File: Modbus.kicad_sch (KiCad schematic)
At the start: 30 parts, among them J4 Term, J5 RS485, J6 RS422, J7 Term, U5 THVD1452DGSR, U6 THVD1452DGSR

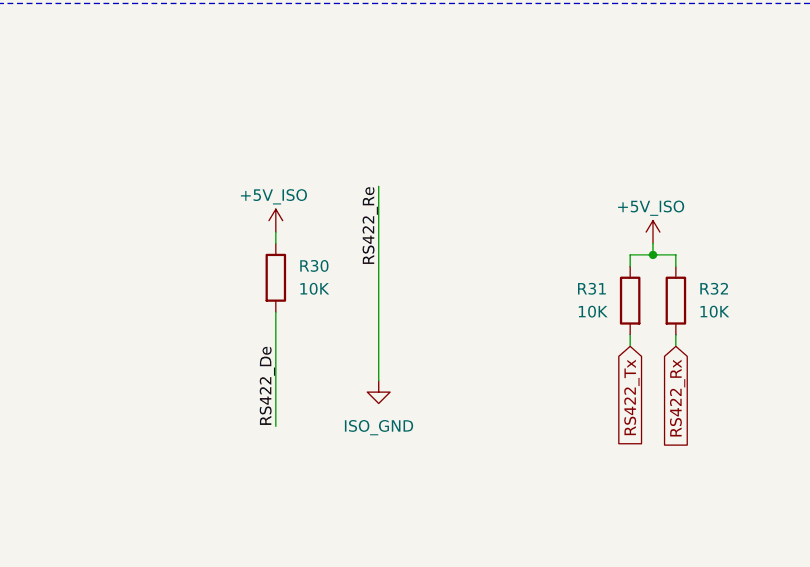
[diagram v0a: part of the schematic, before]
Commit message: reverted back to og files
[local revision r5 4274e03a1d0e]
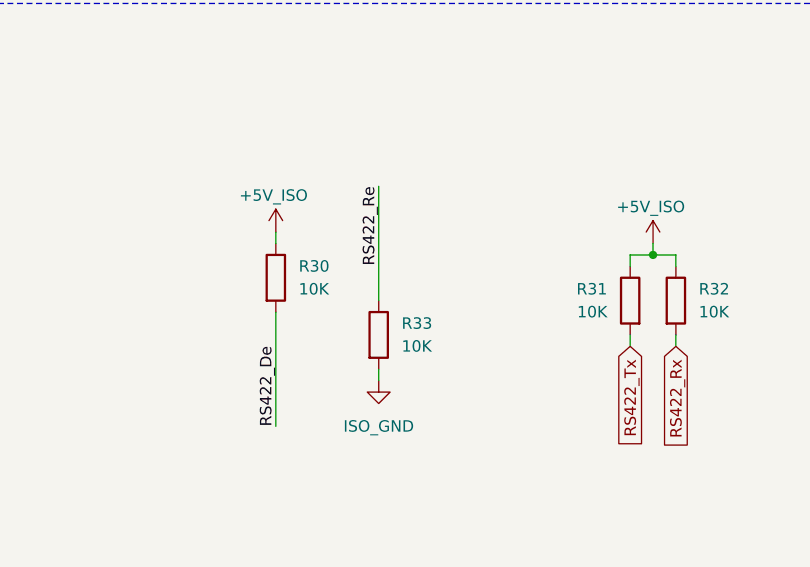
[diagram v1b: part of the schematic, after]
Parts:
- added R33: 10K, Resistor_SMD:R_0805_2012Metric, symbol Device:R
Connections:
- net ISO_GND: now also R33.2; no longer U6.2 (RE)
- new net RS422_Re: R33.1, U6.2 (RE)
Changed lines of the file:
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@@
 	(wire
 		(pts
-			(xy 139.7 113.03) (xy 139.7 134.62)
+			(xy 139.7 133.35) (xy 139.7 134.62)
 		)
 		(stroke
@@
 		(pts
 			(xy 25.4 114.3) (xy 25.4 116.84)
+		)
+		(stroke
+			(width 0)
+			(type default)
+		)
+	)
+	(wire
+		(pts
+			(xy 139.7 125.73) (xy 139.7 113.03)
 		)
 		(stroke
@@
 					(unit 1)
 				)
+			)
+		)
+	)
+	(symbol
+		(lib_id "Device:R")
+		(at 139.7 129.54 0)
+		(unit 1)
+		(body_style 1)
+		(exclude_from_sim no)
+		(in_bom yes)
+		(on_board yes)
+		(in_pos_files yes)
+		(dnp no)
+		(property "Reference" "R33"
+			(at 142.24 128.2699 0)
+			(show_name no)
+			(do_not_autoplace no)
+			(effects
+				(font
+					(size 1.27 1.27)
+				)
+				(justify left)
+			)
+		)
+		(property "Value" "10K"
+			(at 142.24 130.8099 0)
+			(show_name no)
+			(do_not_autoplace no)
+			(effects
+				(font
+					(size 1.27 1.27)
+				)
+				(justify left)
+			)
+		)
+		(property "Footprint" "Resistor_SMD:R_0805_2012Metric"
+			(at 137.922 129.54 90)
+			(hide yes)
+			(show_name no)
+			(do_not_autoplace no)
+			(effects
+				(font
+					(size 1.27 1.27)
+				)
+			)
+		)
+		(property "Datasheet" ""
+			(at 139.7 129.54 0)
+			(hide yes)
+			(show_name no)
+			(do_not_autoplace no)
+			(effects
+				(font
+					(size 1.27 1.27)
+				)
+			)
+		)
+		(property "Description" "Resistor"
+			(at 139.7 129.54 0)
+			(hide yes)
+			(show_name no)
+			(do_not_autoplace no)
+			(effects
+				(font
+					(size 1.27 1.27)
+				)
+			)
+		)
+		(pin "1"
+		)
+		(pin "2"
+		)
+		(instances
+			(project "Demo Project"
+				(path "/4e55511c-c365-4512-9b57-837a9ec6e386/2474e143-7dde-4b68-aaf7-65a89fc37c40"
+					(reference "R33")
+					(unit 1)
+				)

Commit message: testing plugin
[local revision r3 cb60daacd4a3]
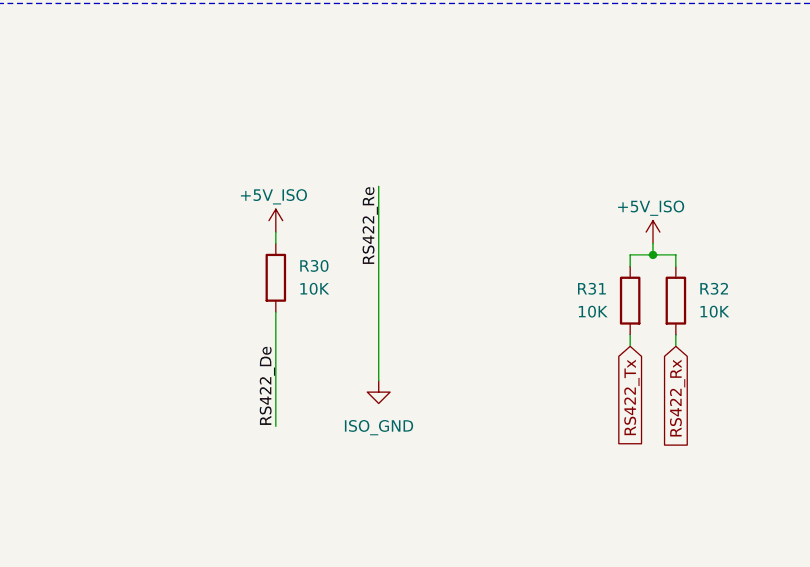
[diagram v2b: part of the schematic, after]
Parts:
- removed R33: 10K, Resistor_SMD:R_0805_2012Metric, symbol Device:R
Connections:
- net RS422_Re is gone; now on net ISO_GND: U6.2 (RE)
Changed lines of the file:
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@@
 	(wire
 		(pts
-			(xy 139.7 133.35) (xy 139.7 134.62)
+			(xy 139.7 113.03) (xy 139.7 134.62)
 		)
 		(stroke
@@
 		(pts
 			(xy 25.4 114.3) (xy 25.4 116.84)
-		)
-		(stroke
-			(width 0)
-			(type default)
-		)
-	)
-	(wire
-		(pts
-			(xy 139.7 125.73) (xy 139.7 113.03)
 		)
 		(stroke
@@
 					(unit 1)
 				)
-			)
-		)
-	)
-	(symbol
-		(lib_id "Device:R")
-		(at 139.7 129.54 0)
-		(unit 1)
-		(body_style 1)
-		(exclude_from_sim no)
-		(in_bom yes)
-		(on_board yes)
-		(in_pos_files yes)
-		(dnp no)
-		(property "Reference" "R33"
-			(at 142.24 128.2699 0)
-			(show_name no)
-			(do_not_autoplace no)
-			(effects
-				(font
-					(size 1.27 1.27)
-				)
-				(justify left)
-			)
-		)
-		(property "Value" "10K"
-			(at 142.24 130.8099 0)
-			(show_name no)
-			(do_not_autoplace no)
-			(effects
-				(font
-					(size 1.27 1.27)
-				)
-				(justify left)
-			)
-		)
-		(property "Footprint" "Resistor_SMD:R_0805_2012Metric"
-			(at 137.922 129.54 90)
-			(hide yes)
-			(show_name no)
-			(do_not_autoplace no)
-			(effects
-				(font
-					(size 1.27 1.27)
-				)
-			)
-		)
-		(property "Datasheet" ""
-			(at 139.7 129.54 0)
-			(hide yes)
-			(show_name no)
-			(do_not_autoplace no)
-			(effects
-				(font
-					(size 1.27 1.27)
-				)
-			)
-		)
-		(property "Description" "Resistor"
-			(at 139.7 129.54 0)
-			(hide yes)
-			(show_name no)
-			(do_not_autoplace no)
-			(effects
-				(font
-					(size 1.27 1.27)
-				)
-			)
-		)
-		(pin "1"
-		)
-		(pin "2"
-		)
-		(instances
-			(project "Demo Project"
-				(path "/4e55511c-c365-4512-9b57-837a9ec6e386/2474e143-7dde-4b68-aaf7-65a89fc37c40"
-					(reference "R33")
-					(unit 1)
-				)
